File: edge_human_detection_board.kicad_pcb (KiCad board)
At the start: 4 copper layers, 58 x 87.5 mm, 20 parts, among them IC1 TXB0108PWR, J1 Conn_01x03_Socket

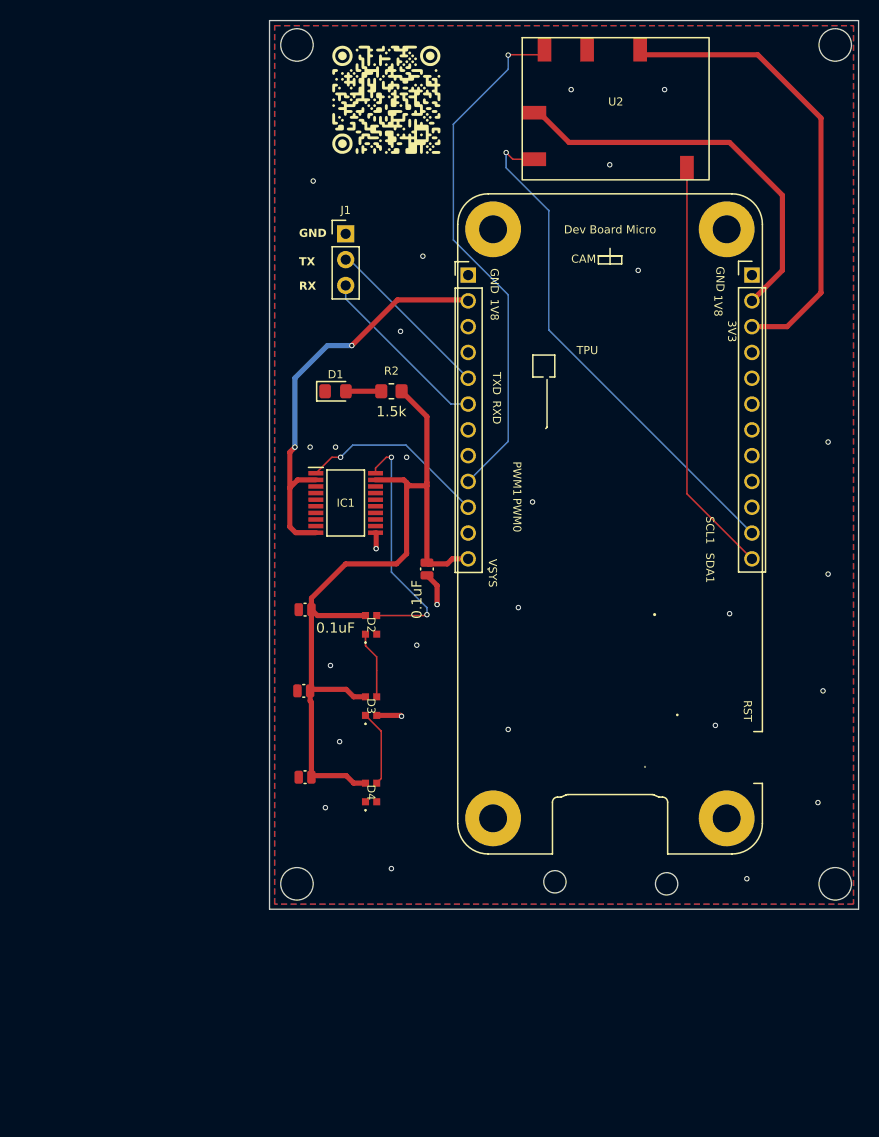
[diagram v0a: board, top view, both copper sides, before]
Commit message: latest updates, up to v2
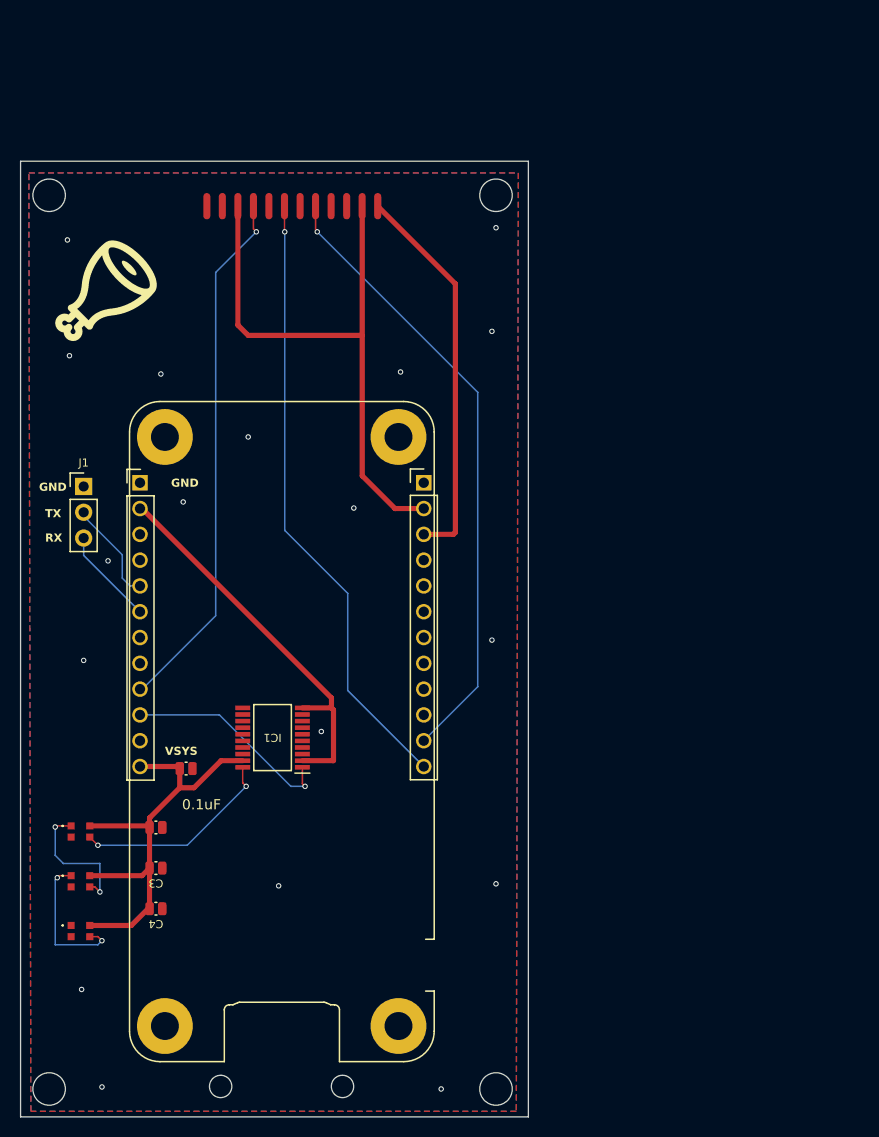
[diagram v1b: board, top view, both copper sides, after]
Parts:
- removed ? (x3): , 
- removed D1: LED, LED_SMD:LED_0805_2012Metric_Pad1.15x1.40mm_HandSolder
- removed R2: 1.5k, Resistor_SMD:R_0805_2012Metric_Pad1.20x1.40mm_HandSolder
- removed the REF** at (142.6, 117.8)
- removed the REF** at (153.6, 118.0)
- removed the REF** at (170.2, 118.0)
- added G***: LOGO, LOGO, F.Cu at (98.4, 59.6)
- added REF**: MountingHole_2.2mm_M2, MountingHole:MountingHole_2.2mm_M2, F.Cu at (109.7, 137.9)
- added REF**: MountingHole_3.2mm_M3, MountingHole:MountingHole_3.2mm_M3, F.Cu at (136.8, 138.2)
- added REF**: MountingHole_3.2mm_M3, MountingHole:MountingHole_3.2mm_M3, F.Cu at (92.8, 138.2)
- added REF**: MountingHole_2.2mm_M2, MountingHole:MountingHole_2.2mm_M2, F.Cu at (121.7, 137.9)
- added REF**: MountingHole_3.2mm_M3, MountingHole:MountingHole_3.2mm_M3, F.Cu at (92.8, 50.2)
- added REF**: MountingHole_3.2mm_M3, MountingHole:MountingHole_3.2mm_M3, F.Cu at (136.8, 50.2)
- G***: moved to B.Cu
- U2: footprint 00_parts_lib:TOF_MODULE -> 00_parts_lib:SATEL-VL53L8A
- moved G*** 84.3 mm to (116.6, 124.6), turned to 180 degrees
- moved U1 38.2 mm to (117.6, 99.6)
- moved J1 35.8 mm to (96.2, 78.9)
- moved U2 35.2 mm to (116.3, 55.5)
- moved D2 35.1 mm to (95.9, 112.8), turned to 180 degrees
- moved D3 33.4 mm to (95.9, 117.7), turned to 180 degrees
- moved D4 31.7 mm to (95.9, 122.6), turned to 180 degrees
- moved C1 30.8 mm to (106.3, 106.6), turned to 180 degrees
- moved C2 26.0 mm to (103.3, 112.4), turned to 180 degrees
- moved IC1 24.2 mm to (114.8, 103.6), turned to 180 degrees
- moved C3 22.7 mm to (103.3, 116.4), turned to 180 degrees
- moved C4 19.6 mm to (103.3, 120.4), turned to 180 degrees
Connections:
- U2 pad 1: /Coral Micro Breakouts/SDA -> GND
- U2 pad 2: /Coral Micro Breakouts/SCL -> unconnected-(U2-NCS-Pad2)
- U2 pad 5: GND -> unconnected-(U2-MISO-Pad5)
- U2 pad 6: /Coral Micro Breakouts/+3.3VDC -> /Coral Micro Breakouts/SDA
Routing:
- net /Coral Micro Breakouts/+5VDC: track 80.5 -> 45.0 mm
- net /Coral Micro Breakouts/+1.8VDC_TOF: track 38.9 -> 58.3 mm
- net /Coral Micro Breakouts/SDA: track 41.7 -> 60.9 mm, vias 0 -> 1
- net /Coral Micro Breakouts/SCL: track 51.2 -> 61.4 mm
- net /Coral Micro Breakouts/DEBUG_RX: track 17.7 -> 9.55 mm
- net GND: track 7.87 -> 0.00 mm, vias 28 -> 18
- net /Coral Micro Breakouts/+3.3VDC: track 45.8 -> 38.5 mm
- net /Coral Micro Breakouts/DEBUG_TX: track 16.9 -> 10.1 mm
- net /RGB Signalling/SIG_IN_RGB3: track 7.50 -> 14.3 mm, vias 0 -> 2
- net /RGB Signalling/SIG_IN_RGB2: track 6.63 -> 13.2 mm, vias 0 -> 2
- net /RGB Signalling/SIG_IN_RGB1: track 24.4 -> 20.1 mm
- net Net-(D1-A): track 3.47 -> 0.00 mm
- net /RGB Signalling/SIG_IN_PWM0: track 18.7 -> 21.1 mm
- net /Coral Micro Breakouts/+1.8VDC_RGB: track 40.7 -> 38.8 mm, vias 2 -> 0
- net /Coral Micro Breakouts/PWM_1: track 51.7 -> 52.5 mm
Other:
- board size 58 x 87.5 mm -> 50 x 94.1 mm
- board text added: "HAAM REV 2.0.0 BY JC"
- board text added: "VSYS"
- board text removed: "EDGE DETECTION BOARD REV 1.1.0 BY JC"
